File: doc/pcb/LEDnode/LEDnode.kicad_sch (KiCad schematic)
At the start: 57 parts, among them J1 LI BAT, Q1 BC807, Q2 BC807, Q3 BC807, Q4 BC807, SW1 EC11J12-15P30C-SW, U1 STM32G071KxT, U2 AF-02841BMR-B, U4 AP1603, U5 BME280, U6 LIS3MDL, Y1 32k768

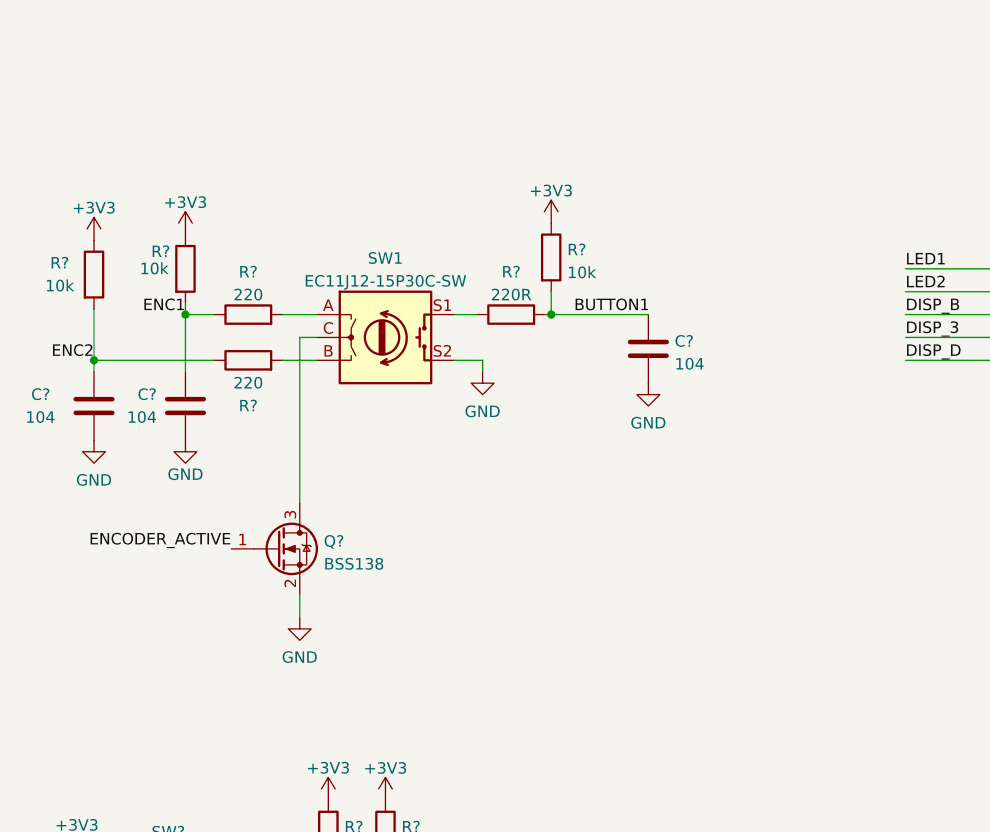
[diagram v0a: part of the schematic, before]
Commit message: almost working menu
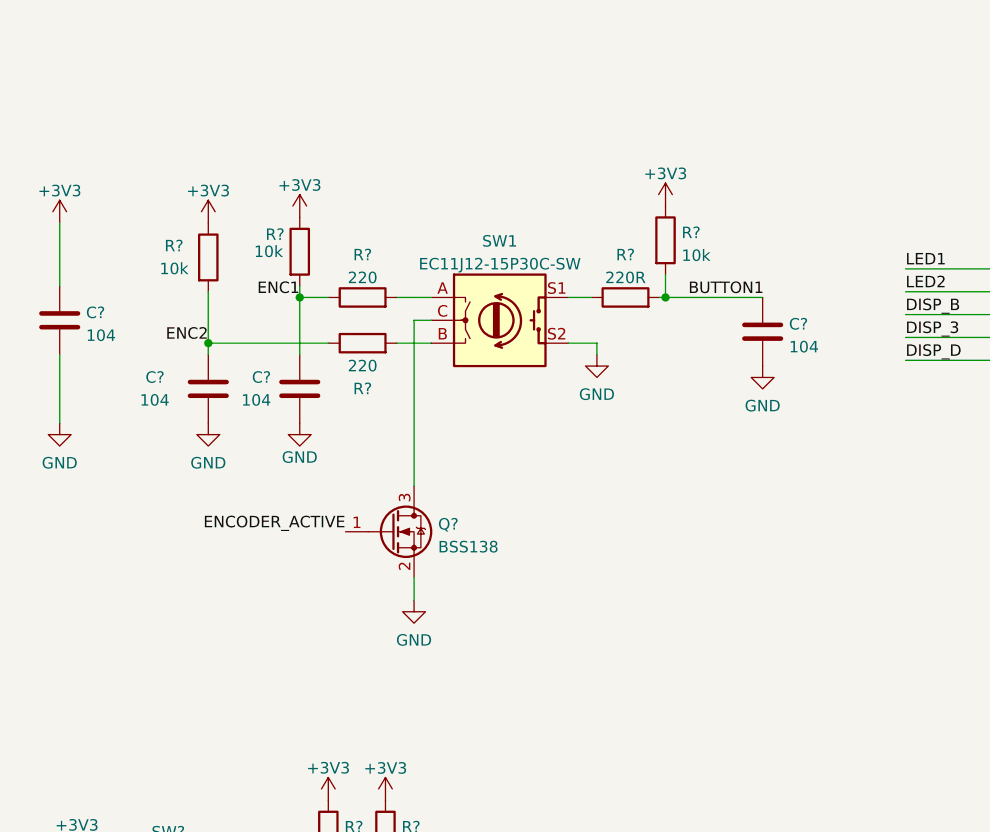
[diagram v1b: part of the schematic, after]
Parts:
- added C?: 104, symbol Device:C
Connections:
- net +3V3: now also C?.1
- net GND: now also C?.2
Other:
- moved on the sheet: C?, Q?, R?, SW1
